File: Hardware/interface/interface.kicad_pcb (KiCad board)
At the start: 2 copper layers, 21 parts, among them J1 TFmini1, J2 TFmini2, J3 TFmini3, U3 TS5A3357, U4 TXB0102DCT, U5 TS5A3357, U6 ARDUINO_MICRO_SHIELD

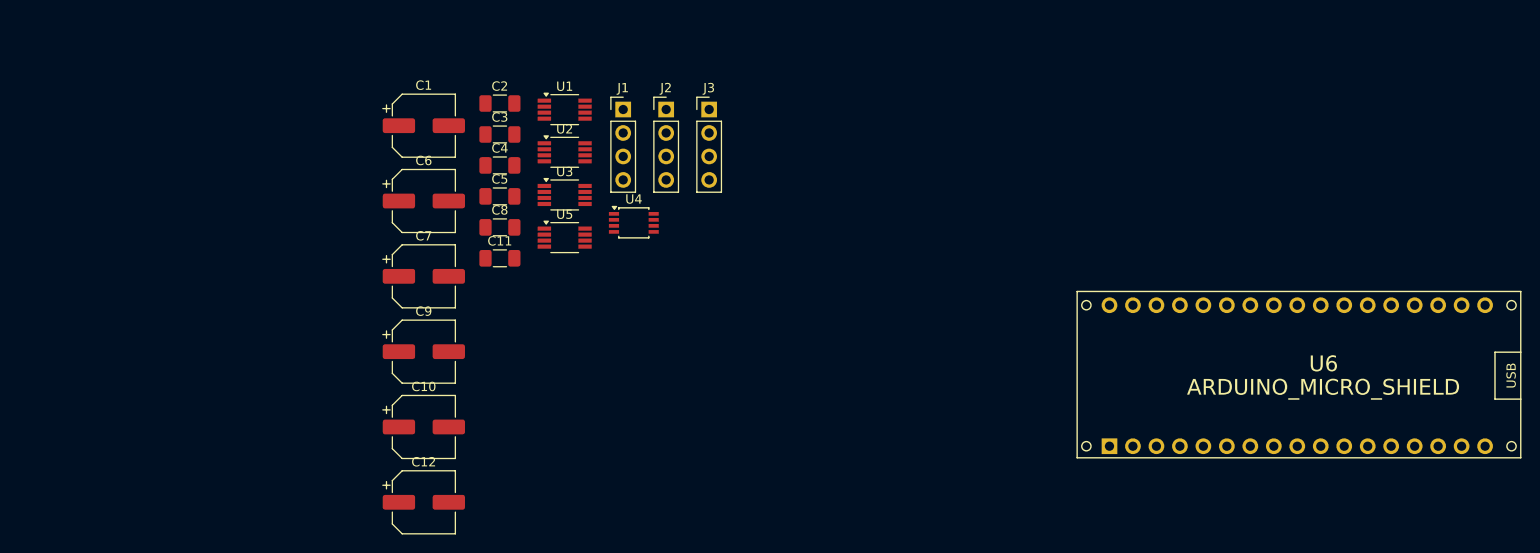
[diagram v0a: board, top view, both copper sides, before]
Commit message: Almost finish PCB routing
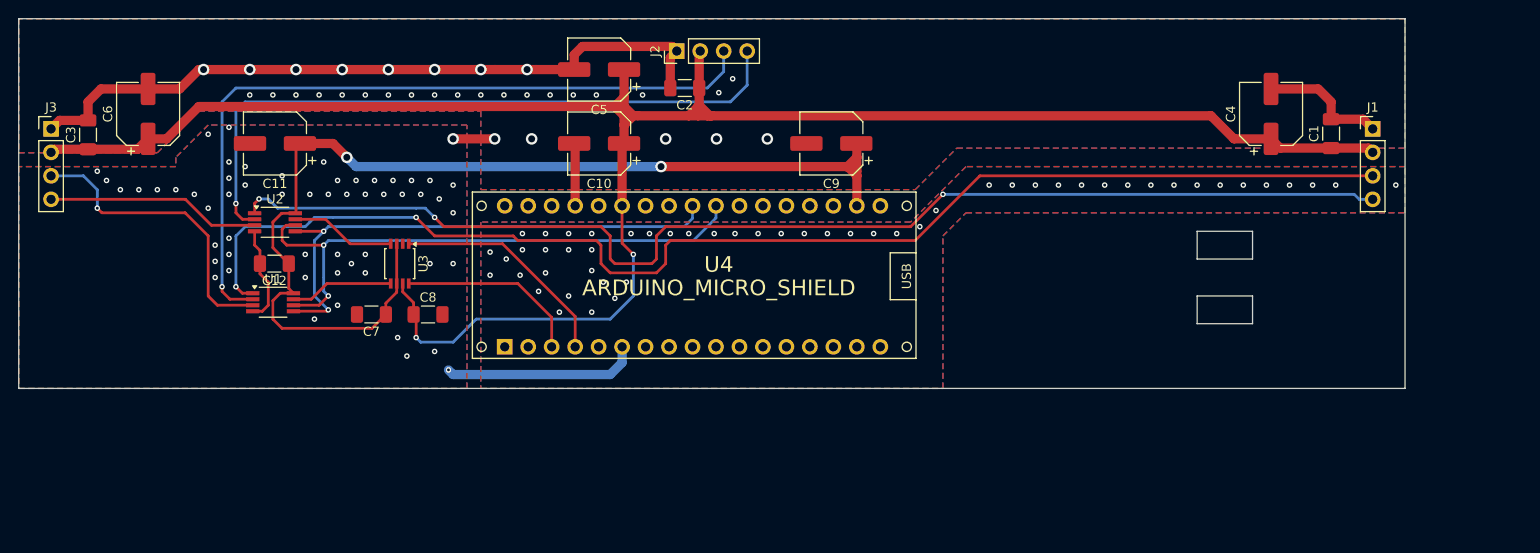
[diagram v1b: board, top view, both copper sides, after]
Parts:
- removed the U3 at (109.1, 69.1)
- removed U5: TS5A3357, Package_SO:VSSOP-8_3.0x3.0mm_P0.65mm
- removed U6: ARDUINO_MICRO_SHIELD, arduino_micro_shield:ARDUINO_MICRO_SHIELD
- added U4: ARDUINO_MICRO_SHIELD, arduino_micro_shield:ARDUINO_MICRO_SHIELD, F.Cu at (99.1, 86.8)
- C1, C12, C7: value 100µF-16V -> 100nF; footprint Capacitor_SMD:CP_Elec_6.3x5.7 -> Capacitor_SMD:C_1206_3216Metric_Pad1.33x1.80mm_HandSolder
- C11, C4, C5: value 100nF -> 100µF-16V; footprint Capacitor_SMD:C_1206_3216Metric_Pad1.33x1.80mm_HandSolder -> Capacitor_SMD:CP_Elec_6.3x5.7
- U1, U2: value ~ -> TS5A3357
- moved C1 98.2 mm to (192.0, 62.4), turned to 90 degrees
- moved C4 83.6 mm to (185.5, 60.3), turned to 90 degrees
- moved J1 81.1 mm to (196.5, 61.9)
- moved J3 71.2 mm to (53.5, 61.9)
- moved C9 49.5 mm to (137.9, 63.5), turned to 180 degrees
- moved C3 44.6 mm to (57.5, 62.6), turned to 90 degrees
- moved U1 37.8 mm to (77.5, 80.7)
- moved C10 36.1 mm to (112.8, 63.5), turned to 180 degrees
- moved U2 32.3 mm to (77.7, 72.0)
- moved C6 31.3 mm to (64.0, 60.3), turned to 90 degrees
- moved C12 30.5 mm to (77.7, 76.5), turned to 180 degrees
- moved C11 27.3 mm to (77.7, 63.5), turned to 180 degrees
- moved U3 25.7 mm to (91.2, 76.5), turned to -90 degrees
- moved C2 20.1 mm to (122.1, 57.5), turned to 180 degrees
- moved C5 17.4 mm to (112.8, 55.5), turned to 180 degrees
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- renumbered U4 to U3
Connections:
- C1 pad 1: +3V3 -> +5V
- C11 pad 1: +5V -> +3V3
- C12 pad 1: +5V -> +3V3
- C2 pad 1: +3V3 -> +5V
- C3 pad 1: +3V3 -> +5V
- C9 pad 1: +5V -> +3V3
- U1 pad 1: (no net) -> /RX_TF1
- U1 pad 2: (no net) -> /RX_TF2
- U1 pad 3: (no net) -> /RX_TF3
- U1 pad 5: (no net) -> /CMD_2
- U1 pad 6: (no net) -> /CMD_1
- U1 pad 7: (no net) -> Net-(U1A-COM)
- U2 pad 1: (no net) -> /TX_TF1
- U2 pad 2: (no net) -> /TX_TF2
- U2 pad 3: (no net) -> /TX_TF3
- U2 pad 5: (no net) -> /CMD_2
- U2 pad 6: (no net) -> /CMD_1
- U2 pad 7: (no net) -> Net-(U2A-COM)
- U3 pad 4: Net-(U4-A2) -> Net-(U2A-COM)
- U3 pad 5: Net-(U3A-COM) -> Net-(U1A-COM)
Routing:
- net +5V: track 0.00 -> 221.7 mm, vias 0 -> 2
- net /RX_TF1: track 0.00 -> 140.6 mm, vias 0 -> 2
- net GND: track 0.00 -> 135.0 mm, vias 0 -> 126
- net /TX_TF1: track 0.00 -> 131.4 mm, vias 0 -> 3
- net +3V3: track 0.00 -> 116.2 mm, vias 0 -> 2
- net /RX_TF2: track 0.00 -> 82.0 mm, vias 0 -> 1
- net /TX_TF2: track 0.00 -> 73.5 mm, vias 0 -> 1
- net /CMD_1: track 0.00 -> 62.4 mm, vias 0 -> 2
- net /CMD_2: track 0.00 -> 58.3 mm, vias 0 -> 2
- net /RX_TF3: track 0.00 -> 32.6 mm, vias 0 -> 1
- net /TX: track 0.00 -> 24.6 mm
- net /TX_TF3: track 0.00 -> 23.2 mm
- net /RX: track 0.00 -> 20.2 mm
- net Net-(U2A-COM): track 0.00 -> 11.4 mm
- net Net-(U1A-COM): track 0.00 -> 11.2 mm
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- added copper zone on B.Cu, net GND
- added copper zone on F.Cu, net GND
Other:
- board outline added: 150 x 40 mm
